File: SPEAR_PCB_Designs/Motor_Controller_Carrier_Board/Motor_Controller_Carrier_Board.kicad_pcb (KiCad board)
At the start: 2 copper layers, 8 parts, among them J1 Conn_01x02_Pin, J2 Conn_01x02_Pin, J3 Conn_01x02_Pin, J4 Conn_01x04_Pin

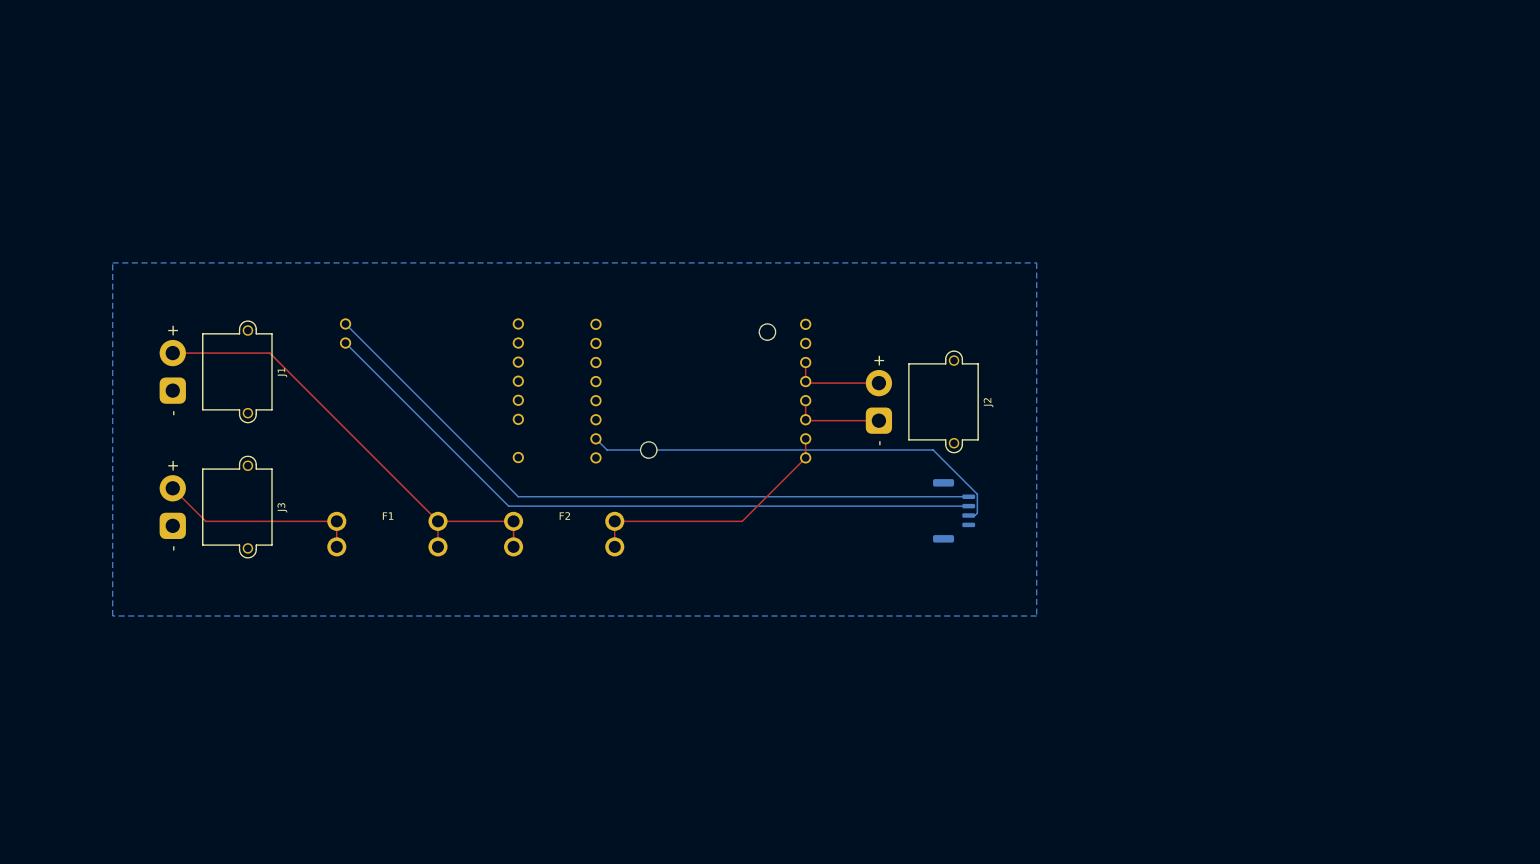
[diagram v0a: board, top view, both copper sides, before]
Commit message: Finished schematic and general PCB layout for carrier board 2992
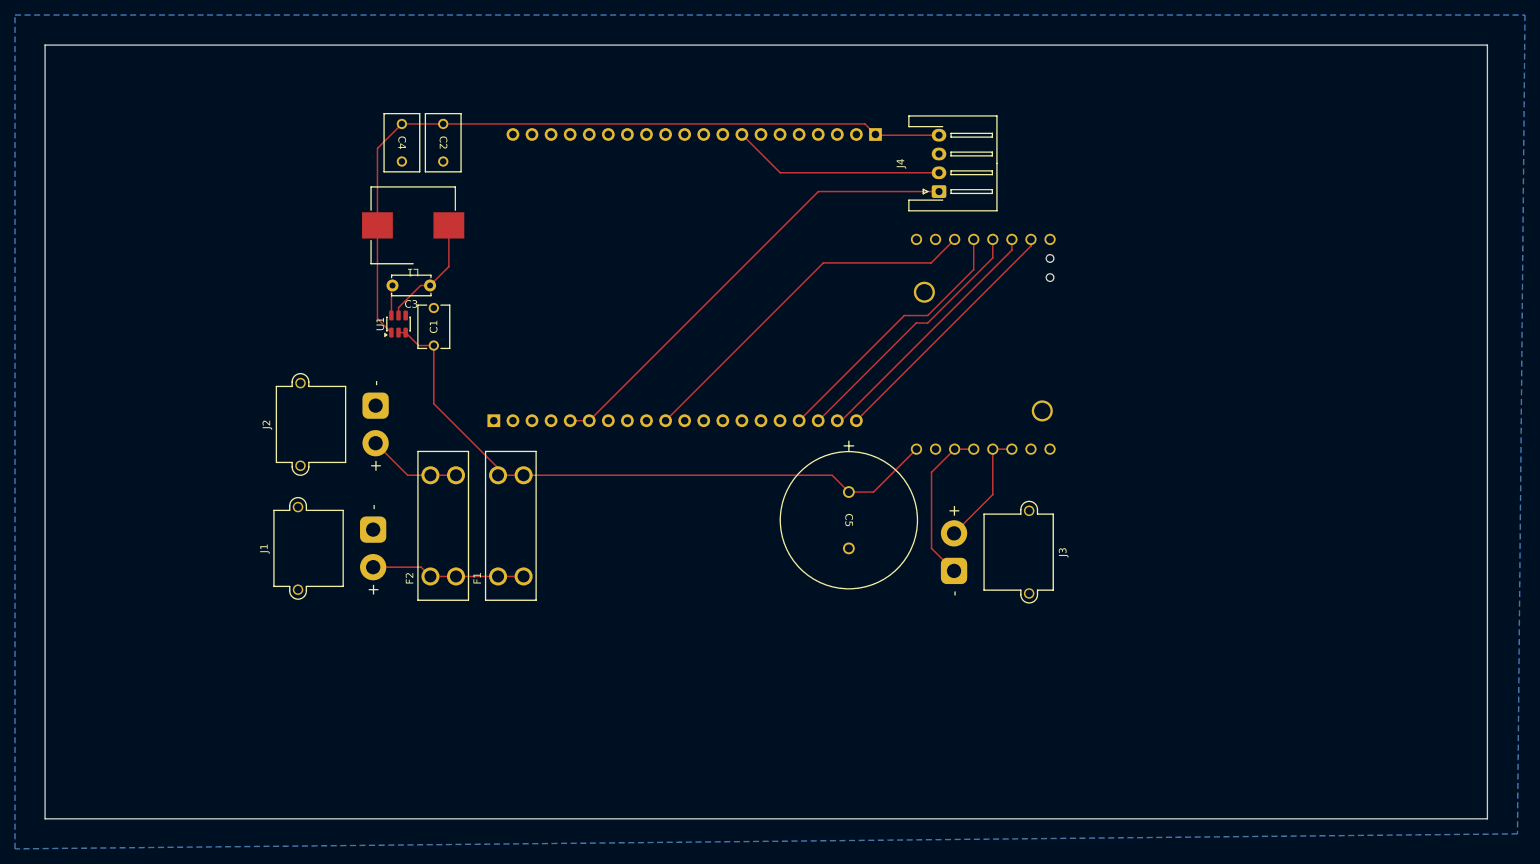
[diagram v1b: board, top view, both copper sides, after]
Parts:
- removed MiCB1: Micro_Controller_Board, SPEAR_Boards:Micro_Controller_Board
- added C1: 10u, SPEAR_AP63203BuckConverter:CAP_FG20_TDK_C1, F.Cu at (106.8, 81.0)
- added C2: 22u, SPEAR_AP63203BuckConverter:CAP_FG22_TDK_C2_C4, F.Cu at (108.0, 51.5)
- added C3: 100n, Capacitor_THT:C_Disc_D5.0mm_W2.5mm_P5.00mm, F.Cu at (106.2, 73.0)
- added C4: 22u, SPEAR_AP63203BuckConverter:CAP_FG22_TDK_C2_C4, F.Cu at (102.5, 51.5)
- added C5: C, Motor_Controller_Carrier_Board:CAP_UBY_18X20_NCH, F.Cu at (162.0, 100.5)
- added L1: 3.9u, SPEAR_AP63203BuckConverter:L_Wurth_WE-LHMI-1040_L1, F.Cu at (104.0, 65.0)
- added MCB1: Micro_Controller_Board, SPEAR_Boards:Micro_Controller_Board, F.Cu at (167.7, 50.0)
- added U1: AP63203WU, Package_TO_SOT_SMD:TSOT-23-6, F.Cu at (102.0, 78.1)
- F1, F2: value Fuse -> 3557-10; footprint Motor_Controller_Carrier_Board:Fuse -> Motor_Controller_Carrier_Board:FUSE_3557-10
- J4: value Conn_01x04_Pin -> JST_S4B-XH-A-1; footprint Motor_Controller_Carrier_Board:JST_GH_BM04B-GHS-TBT_1x04-1MP_P1.25mm_Vertical -> Connector_JST:JST_XH_S4B-XH-A-1_1x04_P2.50mm_Horizontal; moved to F.Cu
- MDB1: value Motor_Driver_Board -> Motor_Driver_Board_2992
- moved J3 104.2 mm to (176.0, 111.0)
- moved J2 67.0 mm to (99.0, 89.0), turned to 90 degrees
- moved MDB1 64.0 mm to (190.1, 65.6), turned to -90 degrees
- moved J4 42.5 mm to (174.0, 60.5), turned to 90 degrees
- moved J1 32.5 mm to (98.7, 105.5), turned to 90 degrees
- moved F1 26.4 mm to (117.0, 105.0), turned to 90 degrees
- moved F2 6.60 mm to (108.0, 105.0), turned to 90 degrees
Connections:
- J2 pad 1: Net-(J2-Pin_1) -> GND
- J3 pad 1: GND -> Net-(J3-Pin_1)
- J4 pad 1: Net-(J4-Pin_1) -> /ENC_B
- J4 pad 2: Net-(J4-Pin_2) -> /ENC_A
- J4 pad 3: Net-(J4-Pin_3) -> GND
- J4 pad 4: GND -> +3.3V
- MDB1 pad 11: Net-(J2-Pin_2) -> Net-(J3-Pin_2)
- MDB1 pad 12: Net-(J2-Pin_2) -> Net-(J3-Pin_2)
- MDB1 pad 13: Net-(J2-Pin_1) -> Net-(J3-Pin_1)
- MDB1 pad 14: Net-(J2-Pin_1) -> Net-(J3-Pin_1)
- MDB1 pad 15: Net-(F2-Pad2) -> +BATT
- MDB1 pad 16: Net-(F2-Pad2) -> +BATT
- MDB1 pad 2: Net-(MDB1-DIR) -> /DIR
- MDB1 pad 3: Net-(MDB1-PWM) -> /PWM
- MDB1 pad 4: Net-(MDB1-SLP) -> /SLP
- MDB1 pad 5: Net-(MDB1-FLT) -> /FLT
- MDB1 pad 6: Net-(MDB1-CS) -> /CS
- MDB1 pad 7: Net-(J4-Pin_3) -> unconnected-(MDB1-3V3-Pad7)
- MDB1 pad 8: Net-(MDB1-VM) -> unconnected-(MDB1-VM-Pad8)
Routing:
- net +3.3V: track 0.00 -> 102.0 mm
- net Net-(J4-Pin_1): track 92.5 -> 0.00 mm
- net Net-(J4-Pin_2): track 91.9 -> 0.00 mm
- net +BATT: track 0.00 -> 85.2 mm
- net /ENC_B: track 0.00 -> 61.7 mm
- net Net-(J4-Pin_3): track 57.6 -> 0.00 mm
- net /CS: track 0.00 -> 48.5 mm
- net Net-(J1-Pin_2): track 61.4 -> 20.5 mm
- net /FLT: track 0.00 -> 35.6 mm
- net Net-(F2-Pad2): track 34.9 -> 0.00 mm
- net /SLP: track 0.00 -> 34.7 mm
- net /PWM: track 0.00 -> 34.1 mm
- net /DIR: track 0.00 -> 33.8 mm
- net /ENC_A: track 0.00 -> 28.4 mm
- net Net-(J3-Pin_1): track 0.00 -> 21.3 mm
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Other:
- board outline added: 192 x 103 mm
